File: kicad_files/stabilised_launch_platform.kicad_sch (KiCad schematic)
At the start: 34 parts, among them J1 Conn_01x03_Male, J2 Conn_01x03_Male, J3 Conn_01x06_Male, J4 USB_C_Receptacle_USB2.0, SW1 SW_Push, U1 MAX7375AXR805, U2 AP7370-33Y, U3 STM32L011F3Px, U4 FT201XS

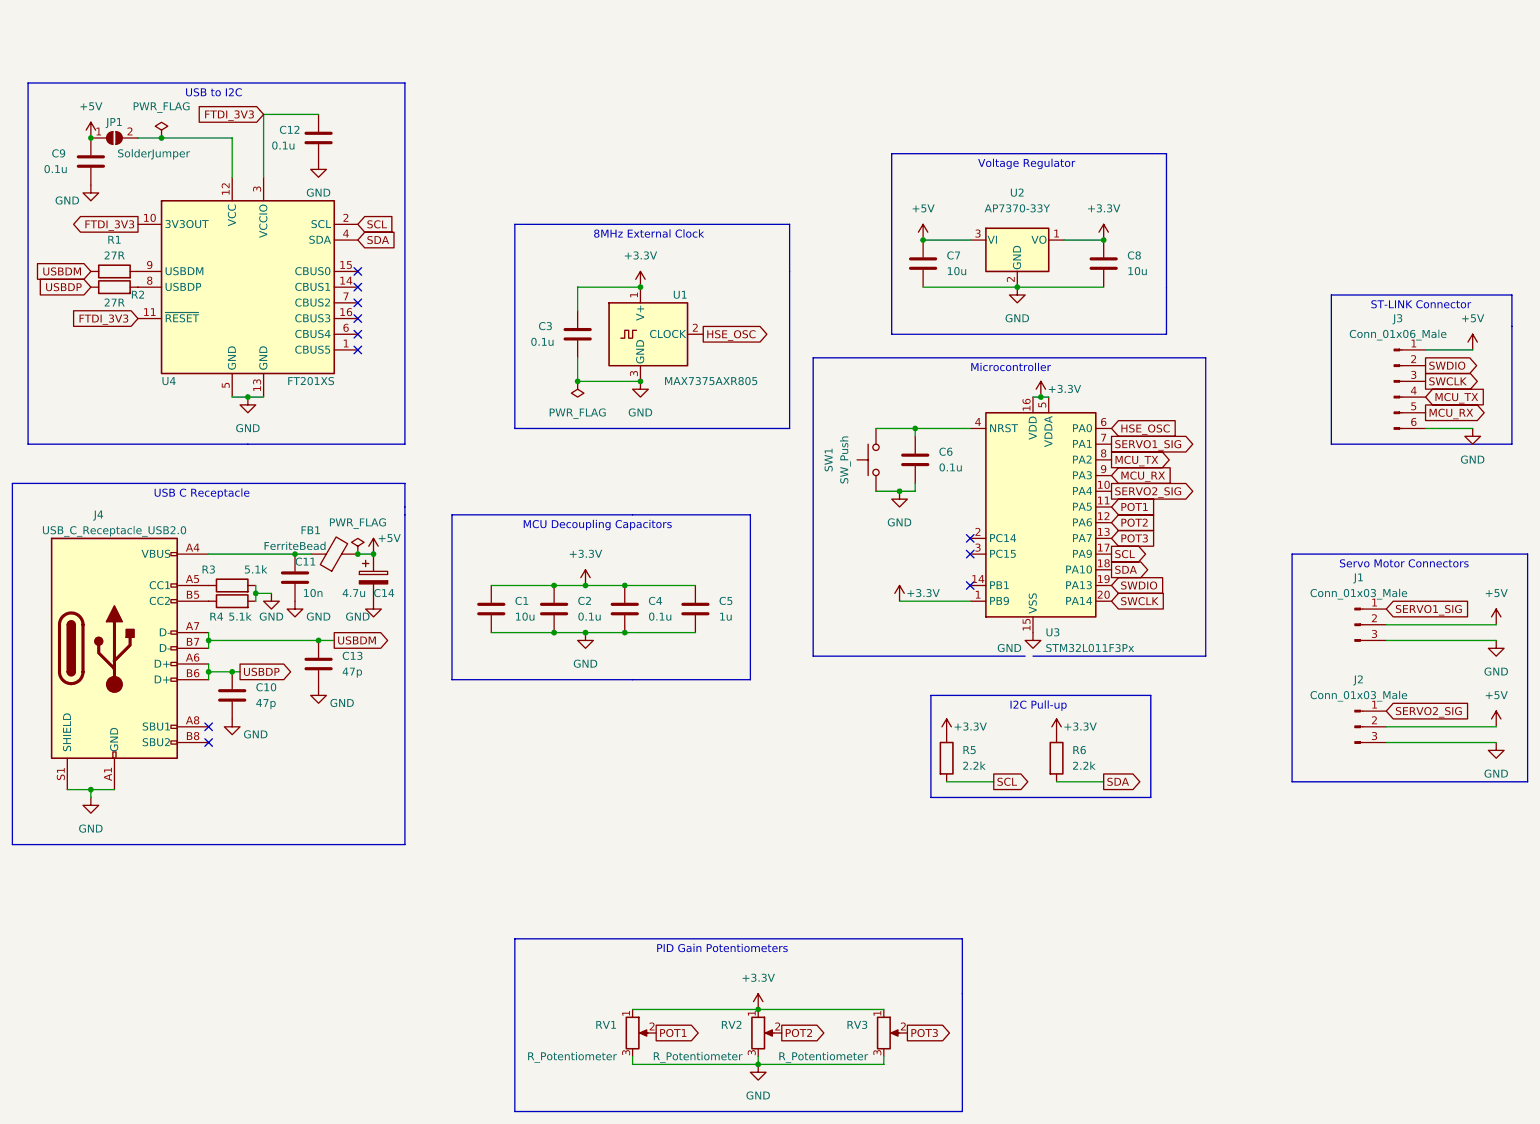
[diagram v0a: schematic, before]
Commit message: Schematic finished
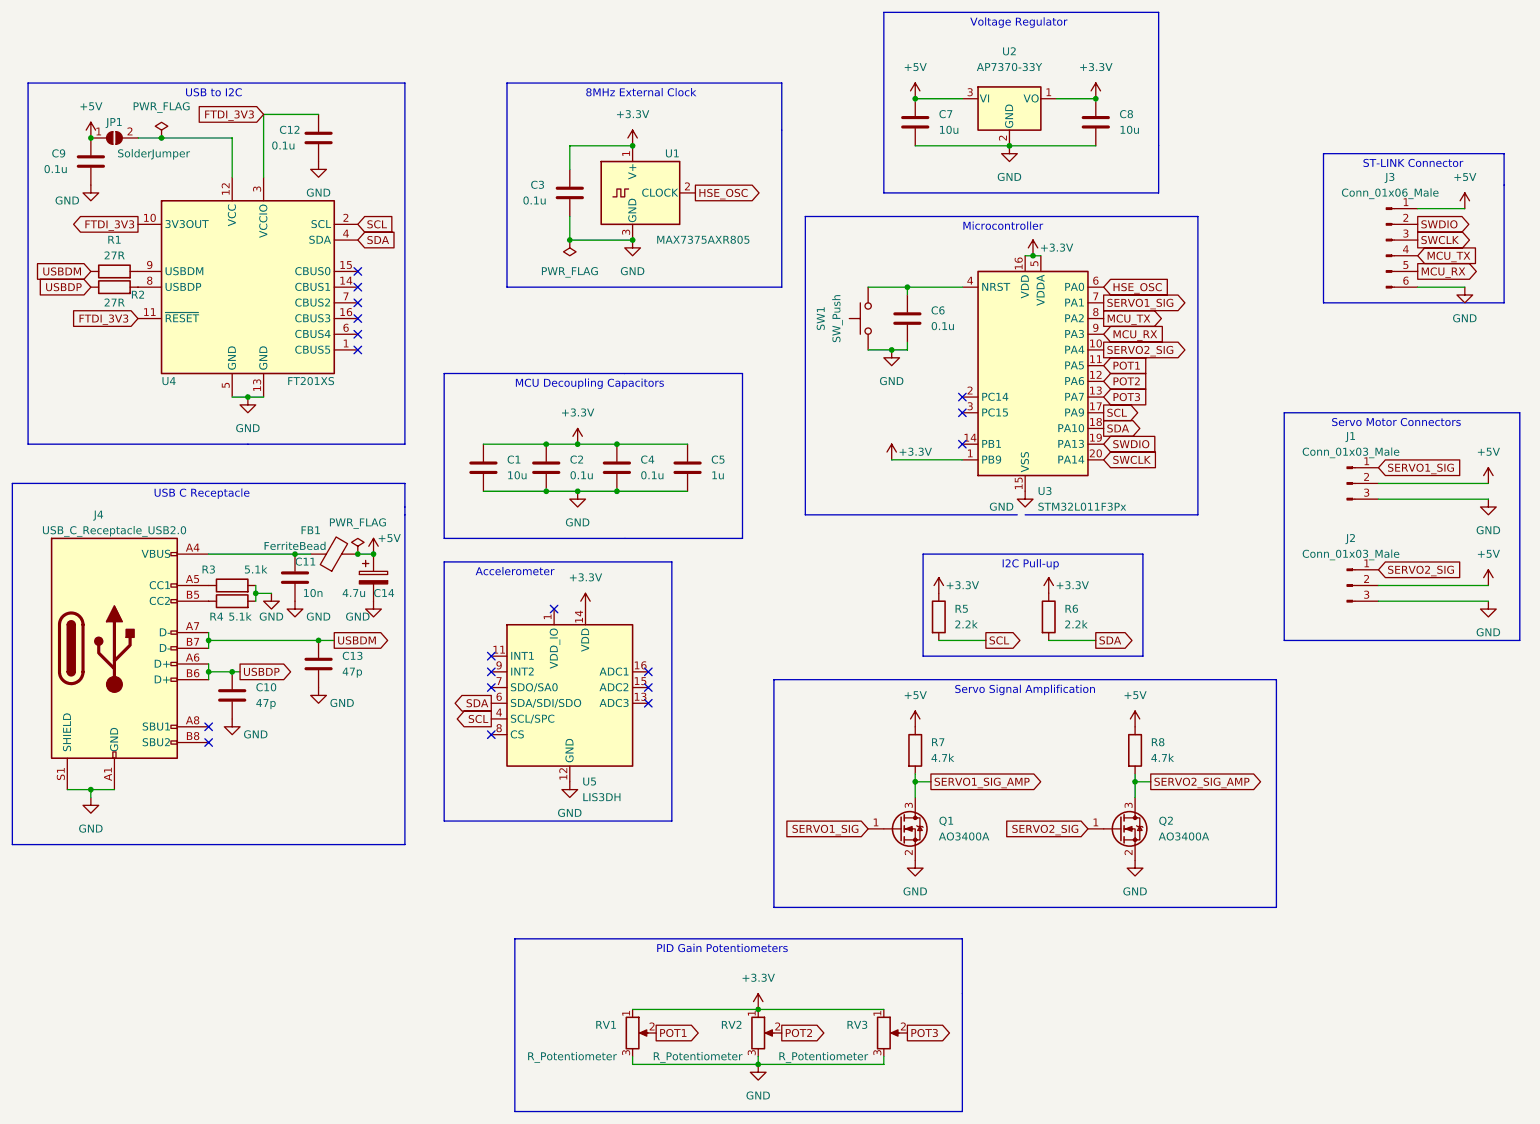
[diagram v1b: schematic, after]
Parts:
- added Q1, Q2: AO3400A, Package_TO_SOT_SMD:SOT-23, symbol Transistor_FET:AO3400A
- added R7, R8: 4.7k, Resistor_SMD:R_0805_2012Metric_Pad1.20x1.40mm_HandSolder, symbol Device:R
- added U5: LIS3DH, Package_LGA:LGA-16_3x3mm_P0.5mm_LayoutBorder3x5y, symbol Sensor_Motion:LIS3DH
- C1, C10, C11, C12, C13, C14, C2, C3, C4, C5, C6, C7, C8, C9: footprint (none) -> Capacitor_SMD:C_0805_2012Metric_Pad1.18x1.45mm_HandSolder
- J1, J2: footprint (none) -> Connector_PinHeader_1.00mm:PinHeader_1x03_P1.00mm_Vertical
- J3: footprint (none) -> Connector_PinHeader_1.00mm:PinHeader_1x06_P1.00mm_Vertical
- J4: footprint (none) -> Connector_USB:USB_C_Receptacle_GCT_USB4085
- R1, R2, R3, R4, R5, R6: footprint (none) -> Resistor_SMD:R_0805_2012Metric_Pad1.20x1.40mm_HandSolder
- RV1, RV2, RV3: footprint (none) -> Potentiometer_THT:Potentiometer_Bourns_PTA4543_Single_Slide
- SW1: footprint (none) -> Button_Switch_SMD:SW_SPST_PTS645
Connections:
- net +3.3V: now also U5.14 (VDD)
- net +5V: now also R7.1, R8.1
- net GND: now also Q1.2 (S), Q2.2 (S), U5.10 (GND), U5.12 (GND), U5.5 (GND)
- net SCL: now also U5.4 (SCL/SPC)
- net SDA: now also U5.6 (SDA/SDI/SDO)
- net SERVO1_SIG: now also Q1.1 (G)
- net SERVO2_SIG: now also Q2.1 (G)
- new net SERVO1_SIG_AMP: Q1.3 (D), R7.2
- new net SERVO2_SIG_AMP: Q2.3 (D), R8.2
- no-connect marks 11 -> 19
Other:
- note added: "Accelerometer"
- note added: "Servo Signal Amplification"
- moved on the sheet: C1, C2, C3, C4, C5, C6, C7, C8, J1, J2, J3, R5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
